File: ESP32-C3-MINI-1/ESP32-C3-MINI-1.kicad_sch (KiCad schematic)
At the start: 19 parts, among them J1 ESP32-C3-DEVKITM-1-J1, J2 ESP32-C3-DEVKITM-1-J2, J3 ESPProg-UART, J4 USB2.0_C, SW1 BOOT, SW2 RESET, U1 ESP32-C3-MINI-1, U2 AMS1117-3.3

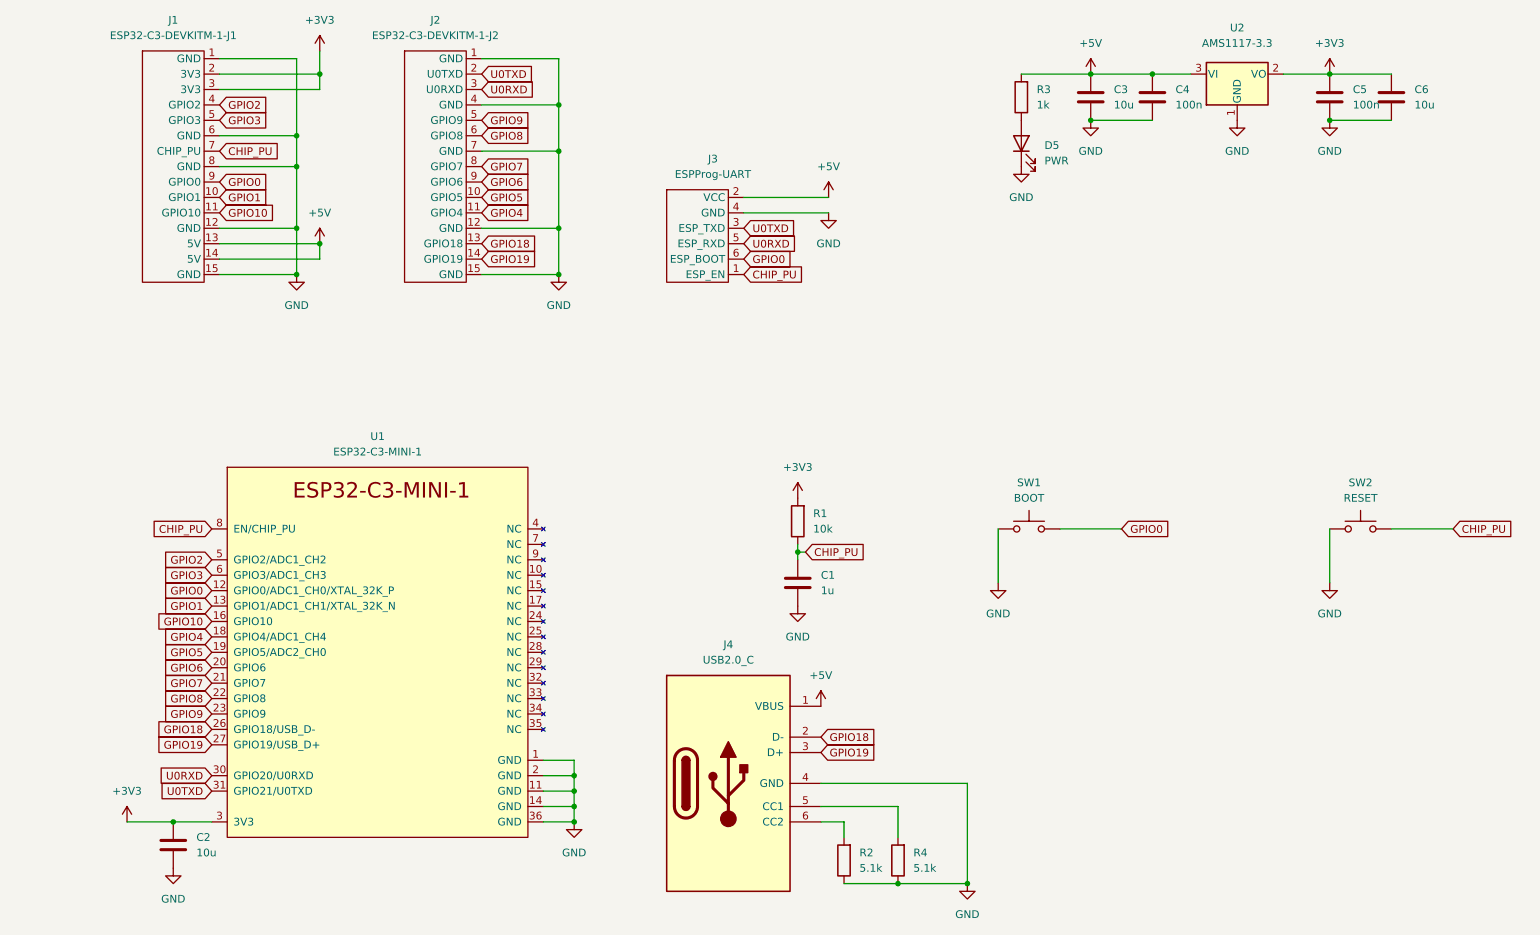
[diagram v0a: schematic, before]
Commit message: before routing
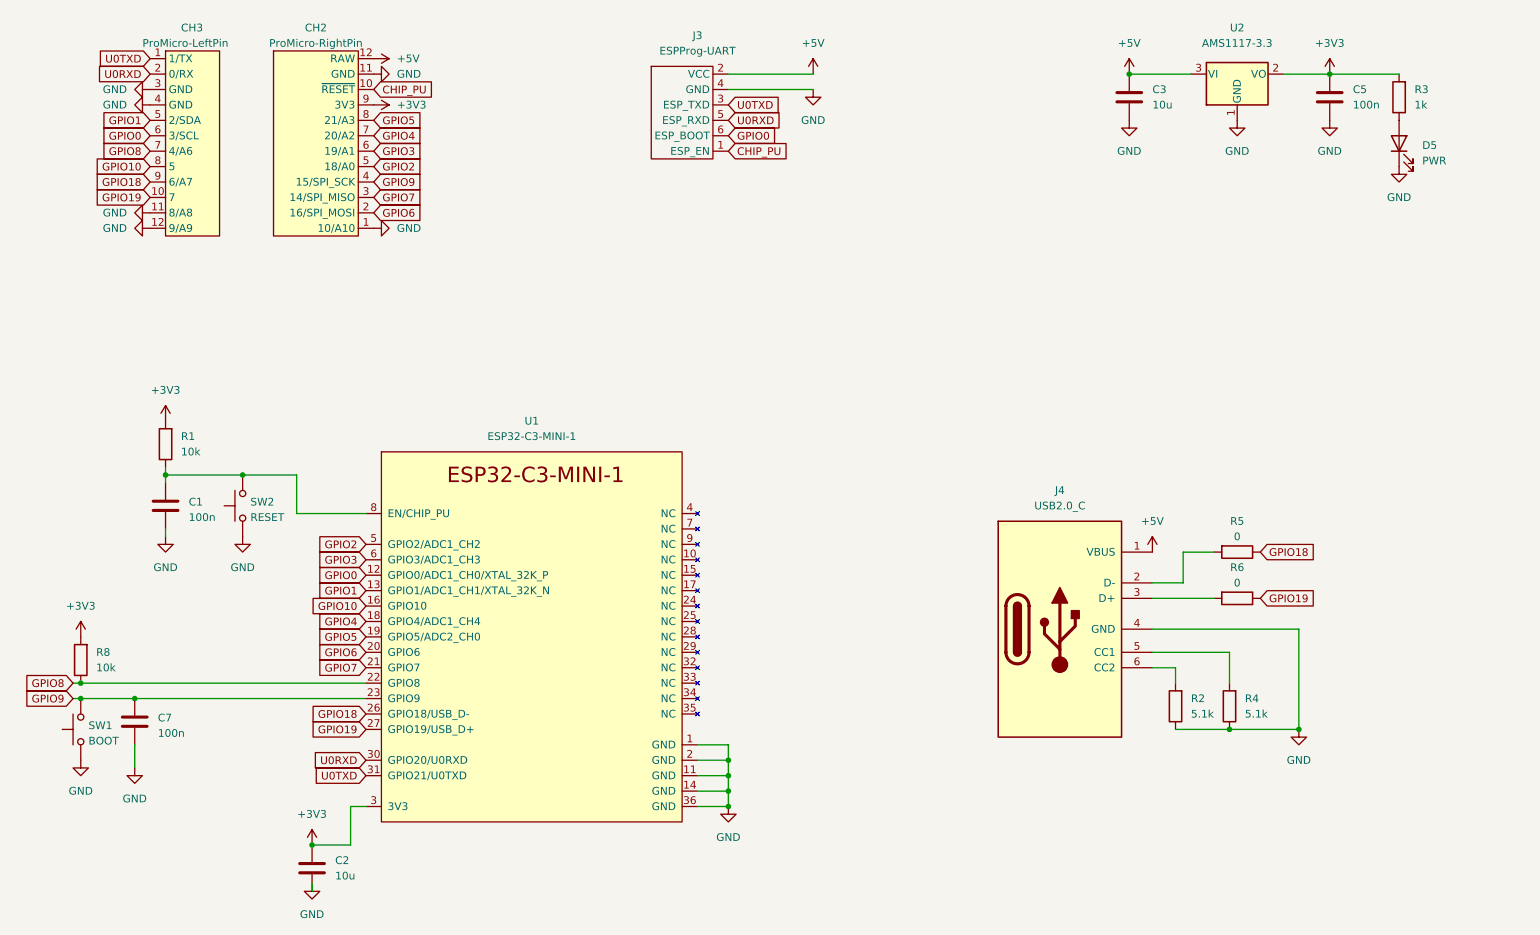
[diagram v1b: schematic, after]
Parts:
- removed C4: 100n, Capacitor_SMD:C_0805_2012Metric_Pad1.18x1.45mm_HandSolder, symbol Device:C
- removed C6: 10u, Capacitor_SMD:C_0805_2012Metric_Pad1.18x1.45mm_HandSolder, symbol Device:C
- removed J1: ESP32-C3-DEVKITM-1-J1, esp32-dev-boards:ESP32-C3-DEVKITM-J1, symbol esp32-dev-boards:ESP32-C3-DEVKITM-1-J1
- removed J2: ESP32-C3-DEVKITM-1-J2, esp32-dev-boards:ESP32-C3-DEVKITM-J2, symbol esp32-dev-boards:ESP32-C3-DEVKITM-1-J2
- added C7: 100n, $74th:Capacitor_0805_2012, symbol Device:C
- added CH2: ProMicro-RightPin, $74th:ProMicro_LIKE_RIGHT, symbol $74th:ProMicro-RightPin
- added CH3: ProMicro-LeftPin, $74th:ProMicro_LIKE_LEFT, symbol $74th:ProMicro-LeftPin
- added R5, R6: 0, $74th:Register_0805_2012, symbol Device:R
- added R8: 10k, $74th:Register_0805_2012, symbol Device:R
- C1: value 1u -> 100n; footprint Capacitor_SMD:C_0805_2012Metric_Pad1.18x1.45mm_HandSolder -> $74th:Capacitor_0805_2012
- C2, C3, C5: footprint Capacitor_SMD:C_0805_2012Metric_Pad1.18x1.45mm_HandSolder -> $74th:Capacitor_0805_2012
- D5: footprint LED_SMD:LED_0805_2012Metric_Pad1.15x1.40mm_HandSolder -> $74th:LED_0805_2012Metric_Pad1.15x1.40mm_HandSolder
- J3: footprint esp32-dev-boards:BoxPinHeader_2x03_P1.27mm_Vertical -> $74th:BoxPinHeader_2x03_P1.27mm_Vertical
- J4: footprint esp32-dev-boards:USB-C-12-Pin-MidMount-ali-v4 -> $74th:USB-C-12-Pin-SMD
- R1, R2, R3, R4: footprint Resistor_SMD:R_0805_2012Metric_Pad1.20x1.40mm_HandSolder -> $74th:Register_0805_2012
- SW1, SW2: footprint esp32-dev-boards:SKRPABE010 -> $74th:SKRPABE010
- U1: footprint Espressif:ESP32-C3-MINI-1_Hand-Soldering -> Espressif:ESP32-C3-MINI-1
- U2: footprint Package_TO_SOT_SMD:SOT-223-3_TabPin2 -> $74th:Regulator_AMS1117_SOT-89
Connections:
- net +3V3: now also R3.2, CH2.9 (3V3), R8.2
- net +5V: now also CH2.12 (RAW); no longer R3.2
- net CHIP_PU: now also CH2.10 (~{RESET}); no longer C1.1, R1.1, SW2.2, U1.8 (EN/CHIP_PU)
- net GND: now also C7.2, CH2.1 (10/A10), CH2.11 (GND), CH3.11 (8/A8), CH3.12 (9/A9), CH3.3 (GND), CH3.4 (GND)
- net GPIO0: now also CH3.6 (3/SCL); no longer SW1.2
- net GPIO1: now also CH3.5 (2/SDA)
- net GPIO10: now also CH3.8 (5)
- net GPIO18: now also CH3.9 (6/A7), R5.1; no longer J4.2 (D-)
- net GPIO19: now also CH3.10 (7), R6.1; no longer J4.3 (D+)
- net GPIO2: now also CH2.5 (18/A0)
- net GPIO3: now also CH2.6 (19/A1)
- net GPIO4: now also CH2.7 (20/A2)
- net GPIO5: now also CH2.8 (21/A3)
- net GPIO6: now also CH2.2 (16/SPI_MOSI)
- net GPIO7: now also CH2.3 (14/SPI_MISO)
- net GPIO8: now also CH3.7 (4/A6), R8.1
- net GPIO9: now also SW1.2, C7.1, CH2.4 (15/SPI_SCK)
- net U0RXD: now also CH3.2 (0/RX)
- net U0TXD: now also CH3.1 (1/TX)
- new net: C1.1, R1.1, SW2.2, U1.8 (EN/CHIP_PU)
- new net: J4.3 (D+), R6.2
- new net: J4.2 (D-), R5.2
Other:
- moved on the sheet: C1, C2, C3, D5, J3, J4, R1, R2, R3, R4, SW1, SW2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
